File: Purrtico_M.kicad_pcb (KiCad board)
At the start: 2 copper layers, 53 parts, among them J2 Conn_01x02, J3 Conn_01x03, J4 Conn_01x02, U1 OPA1679, U2 OPA1679

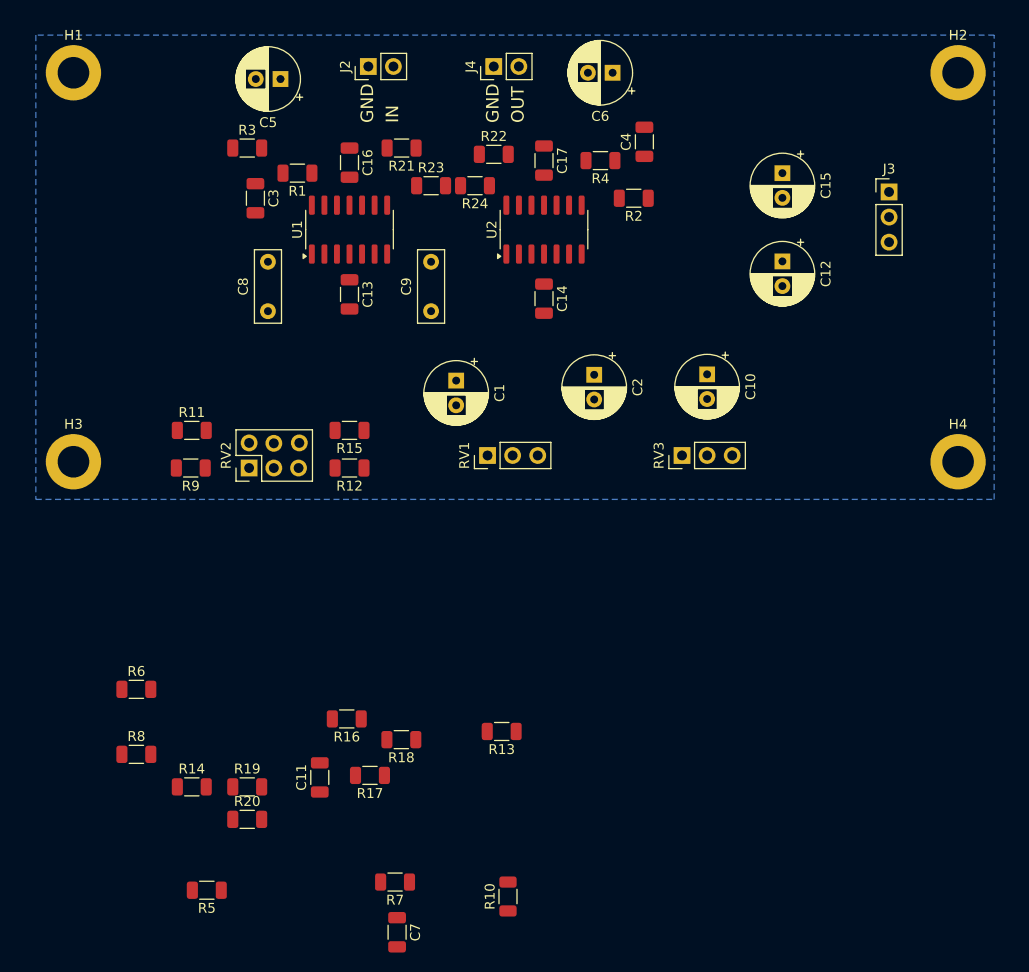
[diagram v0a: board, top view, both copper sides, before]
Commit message: update pcb
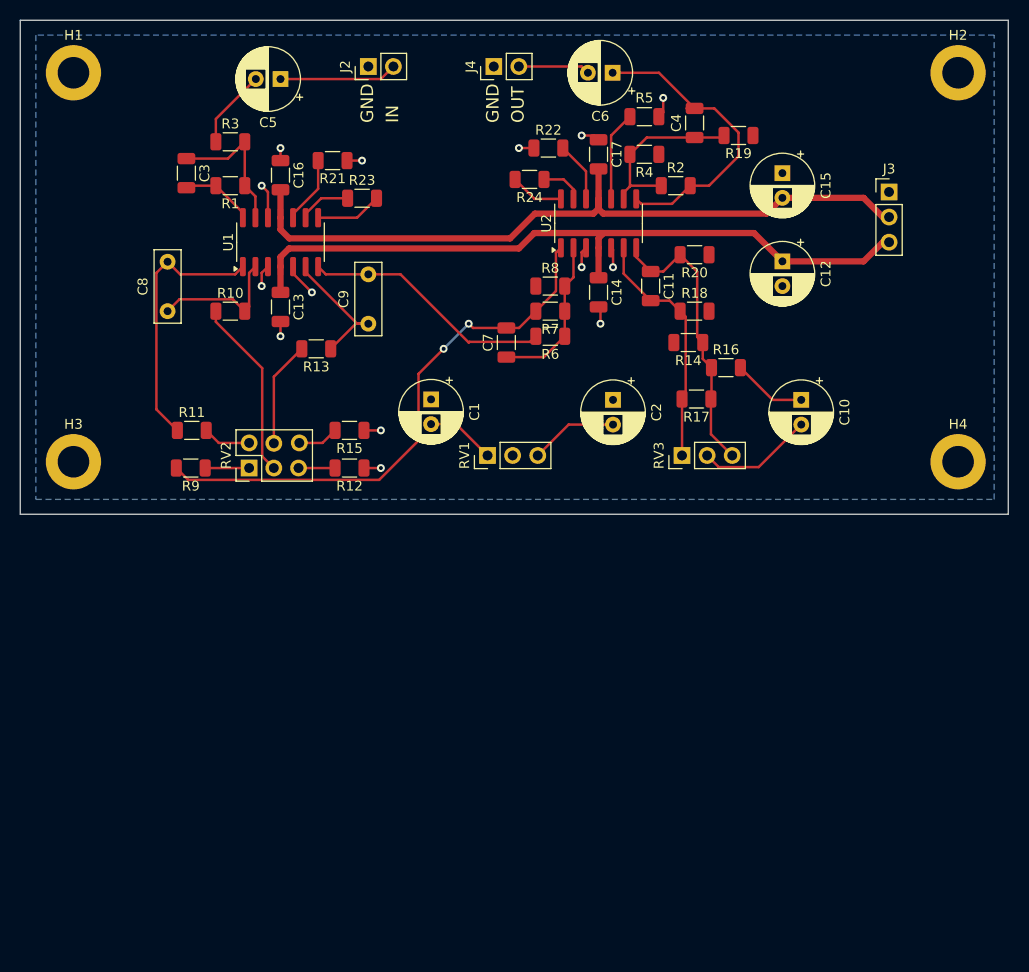
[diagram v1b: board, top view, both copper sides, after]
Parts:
- moved R5 89.9 mm to (150.5, 33.7)
- moved R19 82.6 mm to (160.0, 35.6), turned to 180 degrees
- moved R20 72.9 mm to (155.6, 47.6), turned to 180 degrees
- moved R14 67.4 mm to (154.9, 56.5), turned to 180 degrees
- moved R10 65.6 mm to (108.6, 53.3), turned to 0 degrees
- moved R8 63.3 mm to (141.0, 50.8)
- moved C7 60.7 mm to (136.5, 56.5), turned to 90 degrees
- moved C11 60.0 mm to (151.1, 50.8), turned to -90 degrees
- moved R7 59.9 mm to (141.0, 53.3)
- moved R6 55.1 mm to (141.0, 55.9), turned to 180 degrees
- moved R18 52.6 mm to (155.6, 53.3), turned to 0 degrees
- moved R16 52.3 mm to (158.8, 59.1), turned to 0 degrees
- moved R17 50.4 mm to (155.8, 62.2)
- moved R13 43.0 mm to (117.3, 57.1)
- moved C8 10.2 mm to (102.2, 53.3)
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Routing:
- net -15V: track 0.00 -> 73.9 mm
- net +15V: track 0.00 -> 72.9 mm
- net Net-(C7-Pad2): track 0.00 -> 55.7 mm, vias 0 -> 2
- net Net-(C2-Pad1): track 0.00 -> 31.0 mm
- net Net-(C11-Pad1): track 0.00 -> 29.2 mm
- net GND: track 0.00 -> 28.3 mm, vias 0 -> 14
- net Net-(C8-Pad2): track 0.00 -> 26.9 mm
- net Net-(C9-Pad2): track 0.00 -> 25.5 mm
- net Net-(U2B--): track 0.00 -> 24.9 mm
- net Net-(U2C--): track 0.00 -> 18.5 mm
- net Net-(R10-Pad1): track 0.00 -> 18.3 mm
- net Net-(U2A--): track 0.00 -> 16.1 mm
- net Net-(U1D--): track 0.00 -> 14.7 mm
- net Net-(U1B--): track 0.00 -> 13.9 mm
- net Net-(U1A--): track 0.00 -> 13.8 mm
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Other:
- board outline added: 100 x 50 mm
